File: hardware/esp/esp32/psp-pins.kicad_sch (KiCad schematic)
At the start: 52 parts, among them U1 MCP23008-E/ML, U4 MCP23008-E/ML, U5 MCP42010T-I/SL

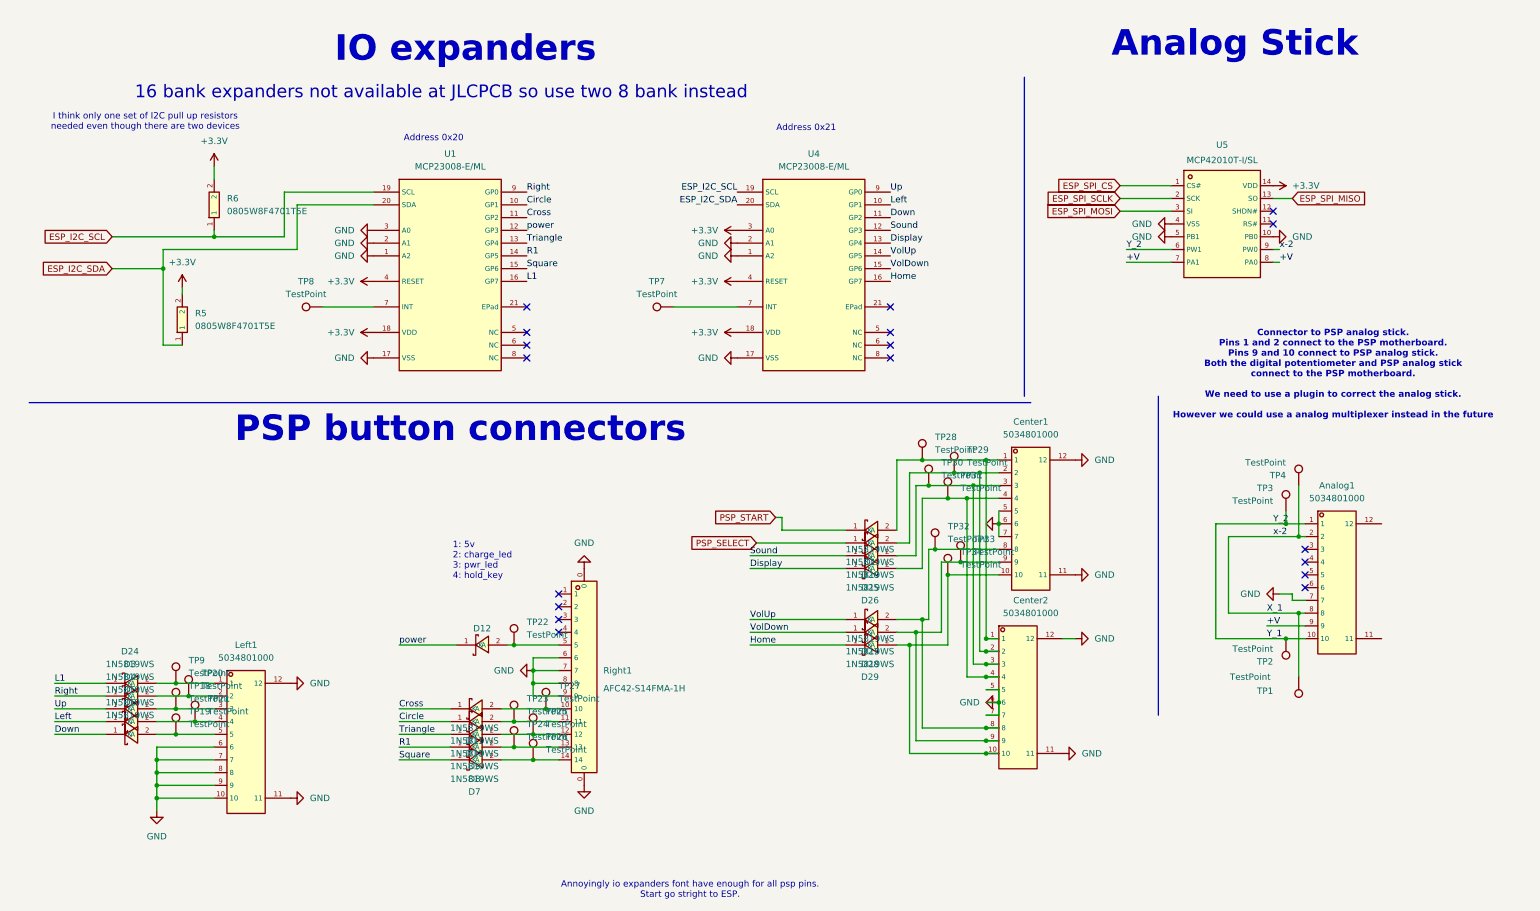
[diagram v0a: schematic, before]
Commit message: wip
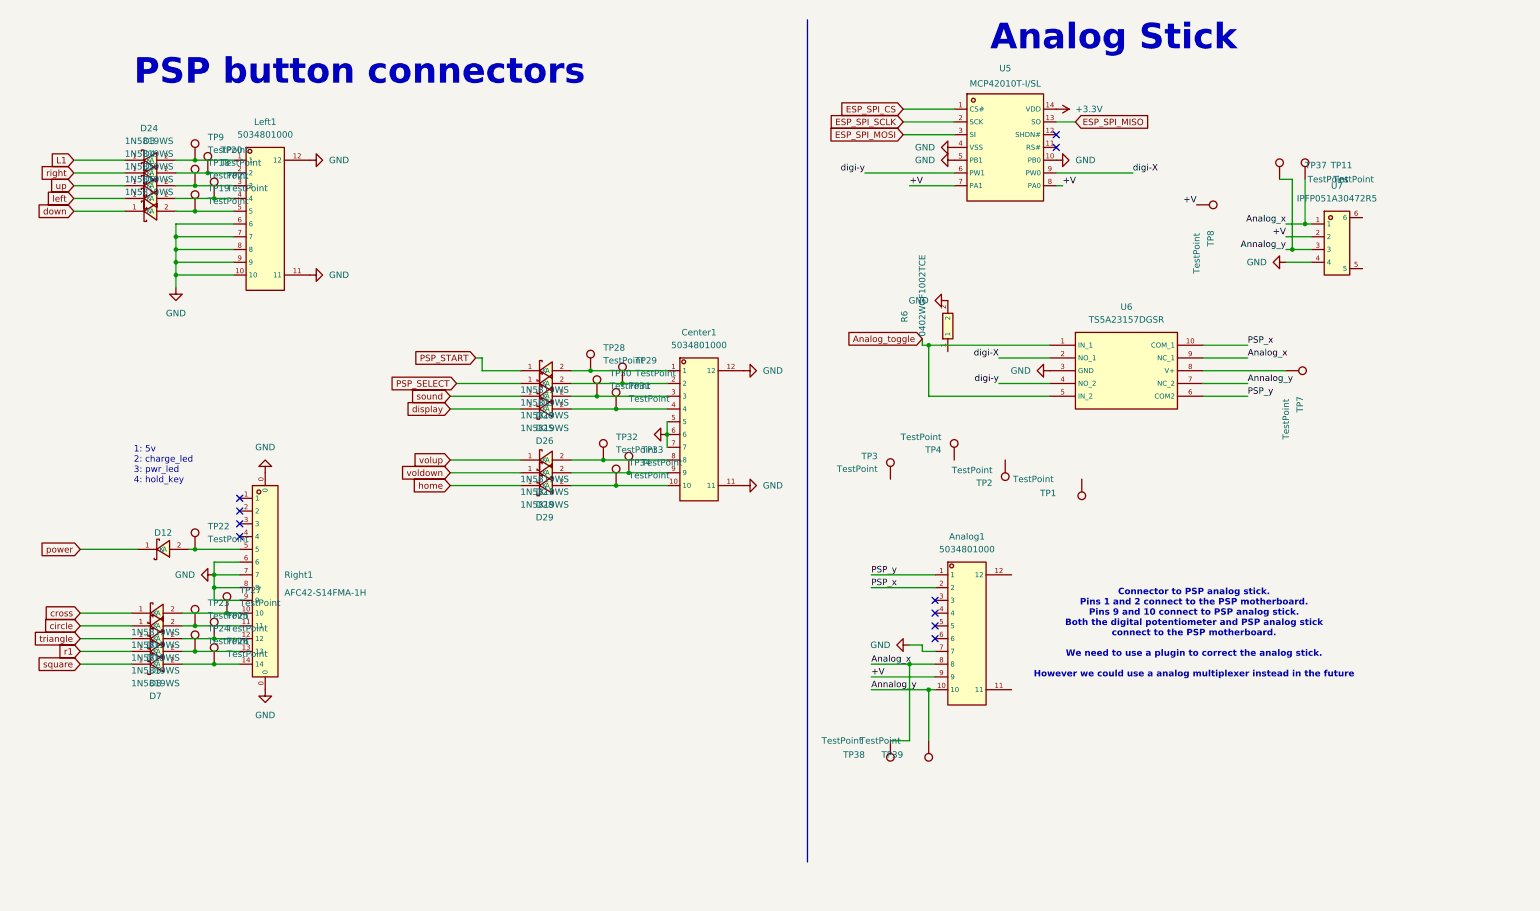
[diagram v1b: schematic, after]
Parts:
- removed Center2: 5034801000, JLCPCB_footprint:FPC-SMD_5034801000, symbol JLCPCB_schematic:5034801000
- removed R5, R6: 0805W8F4701T5E, JLCPCB_footprint:R0805, symbol JLCPCB_schematic:0805W8F4701T5E
- removed U1, U4: MCP23008-E/ML, JLCPCB_footprint:QFN-20_L4.0-W4.0-P0.50-BL-EP2.7, symbol JLCPCB_schematic:MCP23008-E/ML
- added R6: 0402WGF1002TCE, JLCPCB_footprint:R0402, symbol JLCPCB_schematic:0402WGF1002TCE
- added TP11, TP37, TP38, TP39: TestPoint, TestPoint:TestPoint_Pad_D1.0mm, symbol Connector:TestPoint
- added U6: TS5A23157DGSR, JLCPCB_footprint:MSOP-10_L3.0-W3.0-P0.50-LS5.0-BL, symbol JLCPCB_schematic:TS5A23157DGSR
- added U7: IPFP051A30472R5, JLCPCB_footprint:FPC-SMD_4P-P0.50_C9900013912, symbol JLCPCB_schematic:IPFP051A30472R5
- TP7, TP8: footprint TestPoint:TestPoint_Pad_1.5x1.5mm -> TestPoint:TestPoint_Pad_D1.0mm
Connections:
- net +V: now also TP8.1, U7.2
- net GND: now also R6.2, U6.3 (GND), U7.4
- net at TP7.1: now also U6.8 (V+)
- net Circle renamed circle
- net Cross renamed cross
- net Display renamed display
- net Down renamed down
- net Home renamed home
- net Left renamed left
- net R1 renamed r1
- net Right renamed right
- net Sound renamed sound
- net Square renamed square
- net Triangle renamed triangle
- net Up renamed up
- net VolDown renamed voldown
- net VolUp renamed volup
- removed net X_1: Analog1.2, Analog1.8, TP1.1, TP4.1, U5.9 (PW0)
- removed net Y_1: Analog1.1, Analog1.10, TP2.1, TP3.1, U5.6 (PW1)
- new net Analog_toggle: U6.1 (IN_1), U6.5 (IN_2)
- new net Analog_x: Analog1.8, TP11.1, TP38.1, U6.9 (NC_1), U7.1
- new net Annalog_y: Analog1.10, TP37.1, TP39.1, U6.7 (NC_2), U7.3
- new net PSP_x: Analog1.2, U6.10 (COM_1)
- new net PSP_y: Analog1.1, U6.6 (COM2)
- new net digi-X: U5.9 (PW0), U6.2 (NO_1)
- new net digi-y: U5.6 (PW1), U6.4 (NO_2)
- no-connect marks 18 -> 10
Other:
- note removed: "16 bank expanders not available at JLCPCB so use two 8 bank instead"
- note removed: "Address 0x20"
- note removed: "Address 0x21"
- note removed: "Annoyingly io expanders font have enough for all psp pins. Start go stright to ESP."
- note removed: "I think only one set of I2C pull up resistors needed even though there are two devices"
- note removed: "IO expanders"
- moved on the sheet: Analog1, Center1, D1, D10, D11, D12, D20, D24, D25, D26, D27, D28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
